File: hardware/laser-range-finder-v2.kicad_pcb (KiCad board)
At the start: 2 copper layers, 48.2 x 35 mm, 30 parts, among them P1 CON-SENSOR2, P2 DEBUG, P3 BOOT, P4 JST_GHR_6, U1 XMC1100, U2 DRILL, U3 DRILL, U4 DRILL, U5 DRILL

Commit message: add lidar light sensor to 3d model
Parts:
- added REF**: Lidar_Light, kicad-libraries:Lidar_Light, B.Cu at (134.4, 103.7)
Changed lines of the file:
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@@
     (tracks 244)
     (zones 0)
-    (modules 30)
+    (modules 31)
     (nets 22)
   )
@@
   )
   (layers
-    (0 Vorderseite jumper)
+    (0 Vorderseite jumper hide)
     (31 Rückseite signal)
     (32 B.Adhes user)
@@
   )
   (setup
-    (last_trace_width 0.2)
+    (last_trace_width 0.29972)
     (user_trace_width 0.29972)
     (user_trace_width 0.3)
@@
     (aux_axis_origin 110.45 93.65)
     (grid_origin 110.45 93.65)
-    (visible_elements FFFFFFFF)
+    (visible_elements FFFF7FFF)
     (pcbplotparams
       (layerselection 0x010fc_ffffffff)
@@
     (pad EP smd rect (at -5.225 0.925) (size 1.5 2.7) (layers Vorderseite F.Paste F.Mask)
       (net 1 GND))
+    (model Connectors/JST_GHR_6.wrl
+      (at (xyz 0 0 0))
+      (scale (xyz 1 1 1))
+      (rotate (xyz 0 0 0))
+    )
   )
   (module C0402E (layer Vorderseite)
@@
       (clearance 0.65024))
   )
+  (module kicad-libraries:Lidar_Light (layer Rückseite)
+    (at 134.45 103.65 180)
+    (fp_text reference REF** (at 0 -0.5 180) (layer B.Fab)
+      (effects (font (size 0.15 0.15) (thickness 0.0375)) (justify mirror))
+    )
+    (fp_text value Lidar_Light (at 0 0.5 180) (layer B.Fab)
+      (effects (font (size 0.15 0.15) (thickness 0.0375)) (justify mirror))
+    )
+    (fp_line (start -24 10) (end 24 10) (layer B.Fab) (width 0.1))
+    (fp_line (start 24 10) (end 24 -10) (layer B.Fab) (width 0.1))
+    (fp_line (start 24 -10) (end -24 -10) (layer B.Fab) (width 0.1))
+    (fp_line (start -24 -10) (end -24 10) (layer B.Fab) (width 0.1))
+    (model Sensors_Detectors/Garmin_LIDAR-Lite_v3.wrl
+      (at (xyz 0 0 0))
+      (scale (xyz 1 1 1))
+      (rotate (xyz 0 0 0))
+    )
+  )
   (gr_line (start 130.75 117.4) (end 138.15 117.4) (angle 90) (layer Edge.Cuts) (width 0.381))

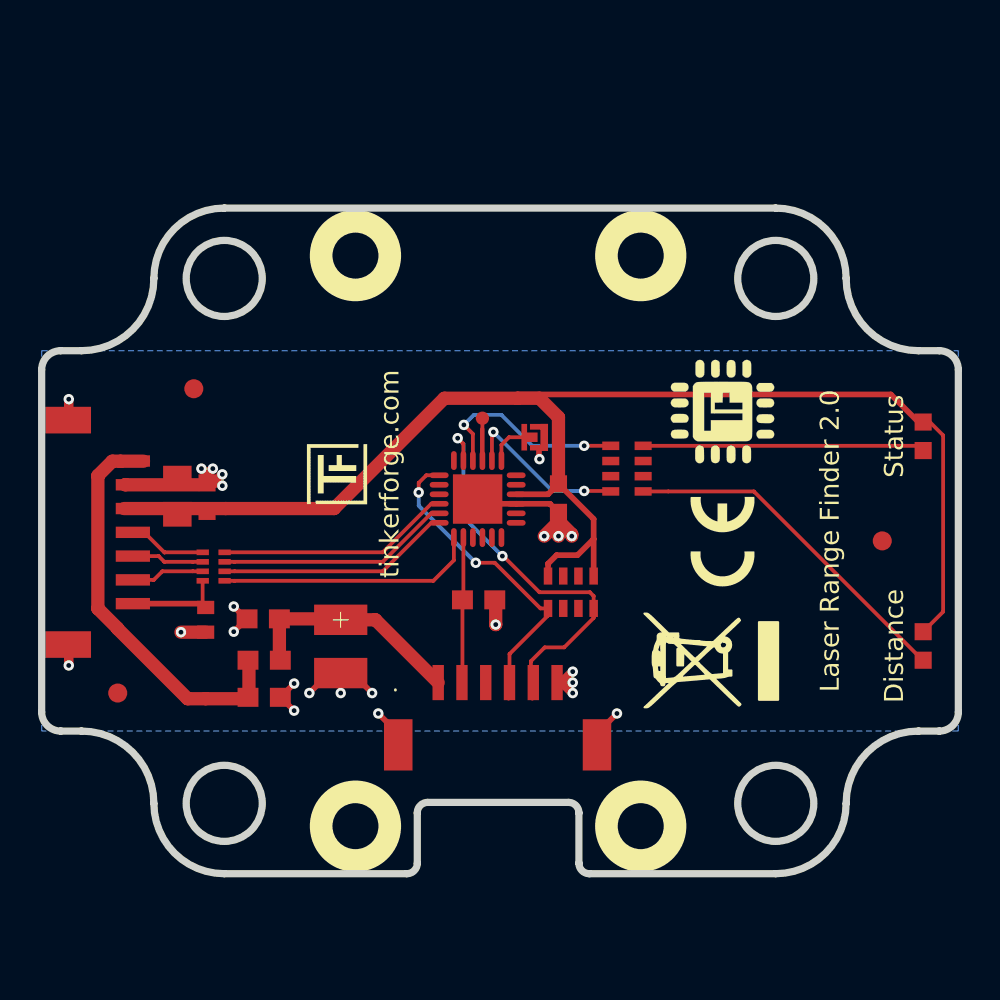
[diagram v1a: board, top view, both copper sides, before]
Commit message: Data Cleanup
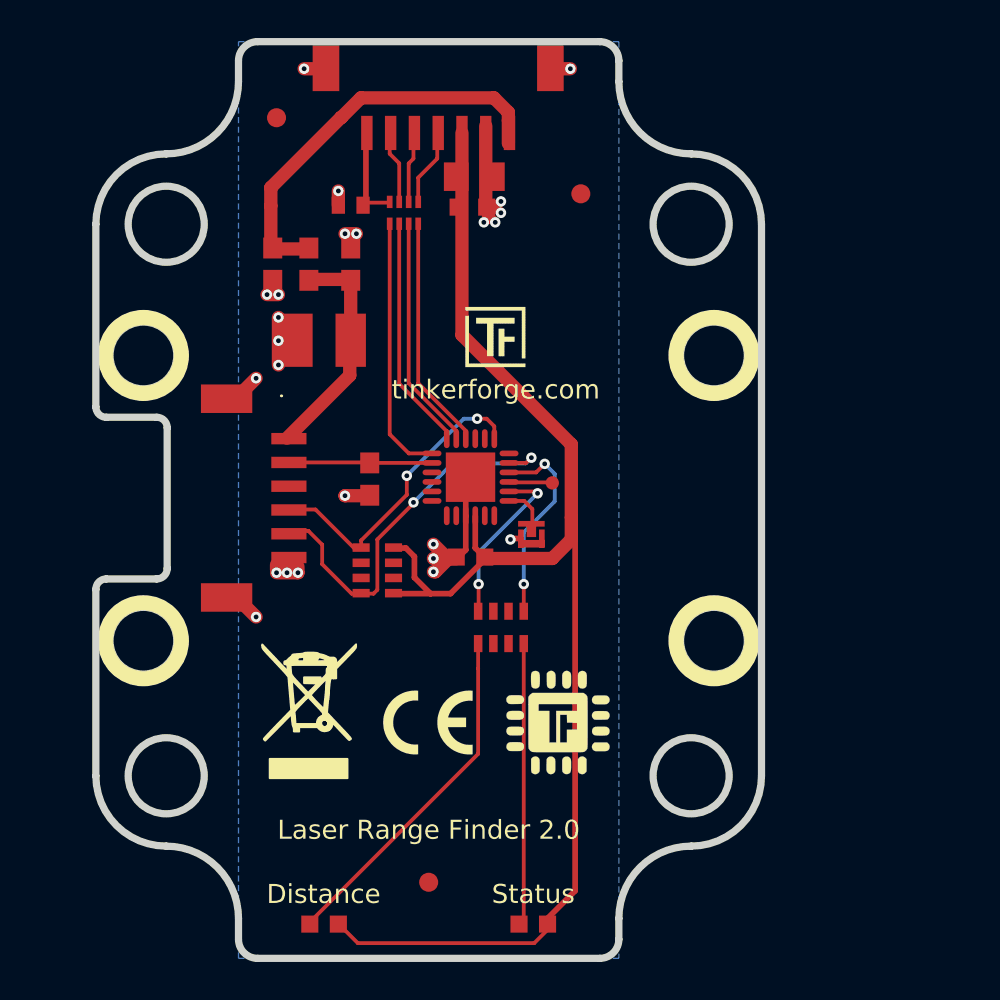
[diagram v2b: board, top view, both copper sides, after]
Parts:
- C7: footprint 3528-21 -> kicad-libraries:3528-21
- U2, U3, U4, U5: footprint DRILL_NP -> kicad-libraries:DRILL_NP
- moved D2 34.7 mm to (125.3, 123.8), turned to 180 degrees
- moved P1 32.9 mm to (131.3, 77.6), turned to 180 degrees
- moved D1 32.8 mm to (136.3, 123.8), turned to 180 degrees
- moved Fiducial_Mark 31.4 mm to (122.8, 81.4), turned to -90 degrees
- moved Fiducial_Mark 29.9 mm to (130.8, 121.6), turned to -90 degrees
- moved U3 27.9 mm to (115.8, 108.9), turned to -90 degrees
- moved U2 27.1 mm to (115.8, 93.9), turned to -90 degrees
- moved C1 23.1 mm to (126.7, 86.0), turned to 180 degrees
- moved C2 22.9 mm to (133.2, 84.5), turned to 0 degrees
- moved Fiducial_Mark 22.8 mm to (138.8, 85.4), turned to -90 degrees
- moved C5 22.8 mm to (122.6, 89.1), turned to -90 degrees
- moved VAL 21.3 mm to (124.5, 112.6), turned to 0 degrees
- moved RP1 21.1 mm to (129.5, 86.4), turned to 180 degrees
- moved L1 21.0 mm to (124.5, 89.1), turned to -90 degrees
- moved C3 20.7 mm to (133.1, 86.1), turned to 0 degrees
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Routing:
- net Net-(P2-Pad1): track 3.90 -> 2.22 mm
- net 3V3: track 75.6 -> 74.6 mm
- net SDA: track 21.6 -> 20.6 mm
- net SCL: track 16.9 -> 16.2 mm
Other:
- board size 48.2 x 35 mm -> 35 x 48.2 mm
- net class Default removed
- board text added: "Copyright Tinkerforge GmbH 2023. This documentation describes Open Hardware and is licensed under the CERN OHL v. 1.1. You may redistribute and modify this documentation under the terms of the CERN OHL v.1.1. (http://ohwr.org/cernohl). This documentation is distributed WITHOUT ANY EXPRESS OR IMPLIED WARRANTY, INCLUDING OF MERCHANTABILITY, SATISFACTORY QUALITY AND FITNESS FOR A PARTICULAR PURPOSE.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"
